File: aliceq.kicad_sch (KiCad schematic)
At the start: 180 parts, among them J1 ISP-6, SW1 SW_Push, U1 ATmega32U4-AU, U2 PRTR5V0U2X, Y1 CLK

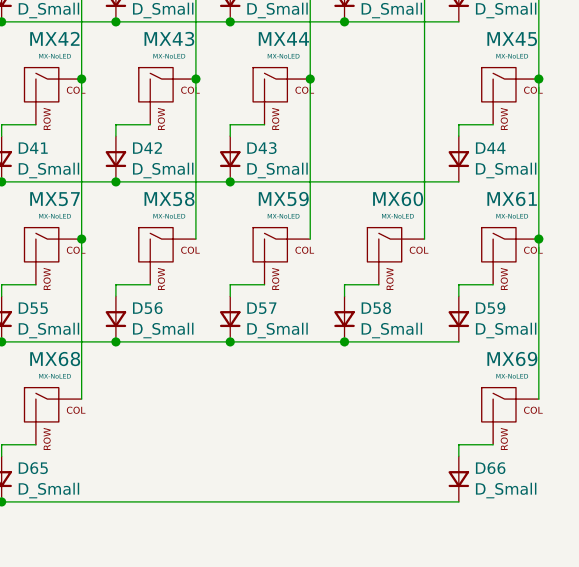
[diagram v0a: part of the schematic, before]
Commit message: More compatibility
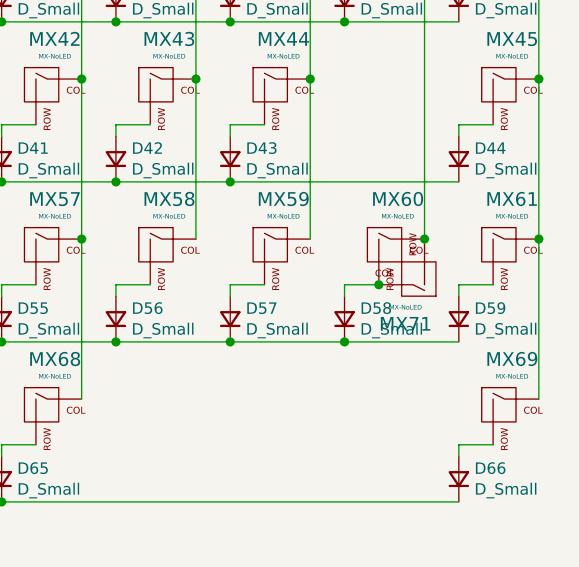
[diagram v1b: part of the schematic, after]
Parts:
- added MX71: MX-NoLED, MX_Only:MXOnly-2.75U-Hotswap-ReversedStabilizers, symbol forty-rescue:MX-NoLED-MX_Alps_Hybrid
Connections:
- net COL13: now also MX71.2 (ROW)
- net at D58.2 (A), MX60.2 (ROW): now also MX71.1 (COL)
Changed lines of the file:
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@@
   (junction (at 251.46 64.77) (diameter 1.016) (color 0 0 0 0))
   (junction (at 251.46 100.33) (diameter 1.016) (color 0 0 0 0))
+  (junction (at 255.27 93.98) (diameter 1.016) (color 0 0 0 0))
   (junction (at 260.35 26.67) (diameter 1.016) (color 0 0 0 0))
   (junction (at 260.35 34.29) (diameter 1.016) (color 0 0 0 0))
   (junction (at 260.35 53.34) (diameter 1.016) (color 0 0 0 0))
+  (junction (at 260.35 88.9) (diameter 1.016) (color 0 0 0 0))
   (junction (at 273.05 34.29) (diameter 1.016) (color 0 0 0 0))
   (junction (at 273.05 53.34) (diameter 1.016) (color 0 0 0 0))
@@
     (pin "2")
   )
+  (symbol (lib_id "forty-rescue:MX-NoLED-MX_Alps_Hybrid") (at 259.08 92.71 180) (unit 1)
+    (in_bom yes) (on_board yes)
+    (property "Reference" "MX71" (id 0) (at 258.2418 98.3742 0)
+      (effects (font (size 1.524 1.524)))
+    )
+    (property "Value" "MX-NoLED" (id 1) (at 258.2418 96.4946 0)
+      (effects (font (size 0.508 0.508)))
+    )
+    (property "Footprint" "MX_Only:MXOnly-2.75U-Hotswap-ReversedStabilizers" (id 2) (at 274.955 92.075 0)
+      (effects (font (size 1.524 1.524)) hide)
+    )
+    (property "Datasheet" "" (id 3) (at 274.955 92.075 0)
+      (effects (font (size 1.524 1.524)) hide)
+    )
+    (pin "1")
+    (pin "2")
+  )
   (symbol (lib_id "forty-rescue:MX-NoLED-MX_Alps_Hybrid") (at 269.24 35.56 0) (unit 1)
     (in_bom yes) (on_board yes)
@@
       (reference "MX70") (unit 1) (value "MX-NoLED") (footprint "MX_Only:MXOnly-1.25U-Hotswap")
     )
+    (path "/13373f14-5dcc-4b9b-80cc-eac714d4bb53"
+      (reference "MX71") (unit 1) (value "MX-NoLED") (footprint "MX_Only:MXOnly-2.75U-Hotswap-ReversedStabilizers")
+    )
     (path "/00000000-0000-0000-0000-00005fe7643d"
